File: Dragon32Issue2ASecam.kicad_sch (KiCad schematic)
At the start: 1 part

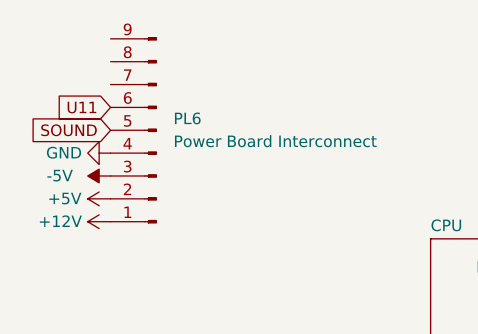
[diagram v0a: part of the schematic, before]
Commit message: fm circuit routing
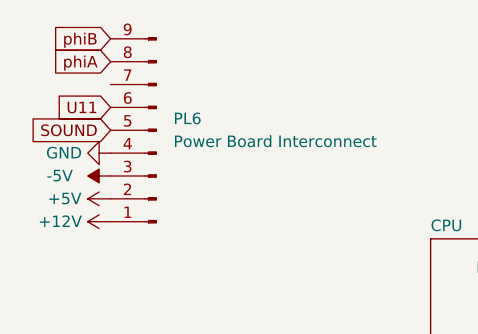
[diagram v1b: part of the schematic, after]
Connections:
- net phiA: now reaches PL6.8 (Pin_8)
- net phiB: now reaches PL6.9 (Pin_9)
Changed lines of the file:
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@@
+		)
+	)
+	(global_label "phiB"
+		(shape input)
+		(at 33.02 22.86 180)
+		(fields_autoplaced yes)
+		(effects
+			(font
+				(size 1.27 1.27)
+			)
+			(justify right)
+		)
+		(property "Intersheetrefs" "${INTERSHEET_REFS}"
+			(at 25.862 22.86 0)
+			(effects
+				(font
+					(size 1.27 1.27)
+				)
+				(justify right)
+				(hide yes)
+			)
 		)
 	)
@@
 			(effects
 				(font
+					(size 1.27 1.27)
+				)
+				(justify right)
+				(hide yes)
+			)
+		)
+	)
+	(global_label "phiA"
+		(shape input)
+		(at 33.02 25.4 180)
+		(fields_autoplaced yes)
+		(effects
+			(font
+				(size 1.27 1.27)
+			)
+			(justify right)
+		)
+		(property "Intersheetrefs" "${INTERSHEET_REFS}"
+			(at 26.0434 25.4 0)
+			(effects
+				(font

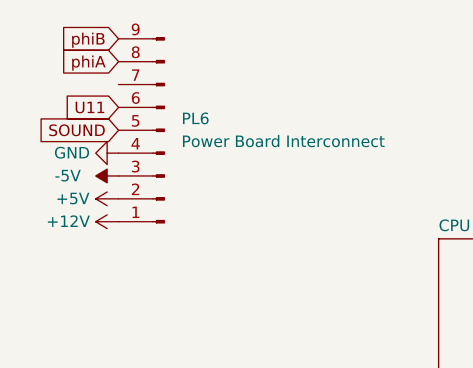
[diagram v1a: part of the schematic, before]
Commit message: trace work complete
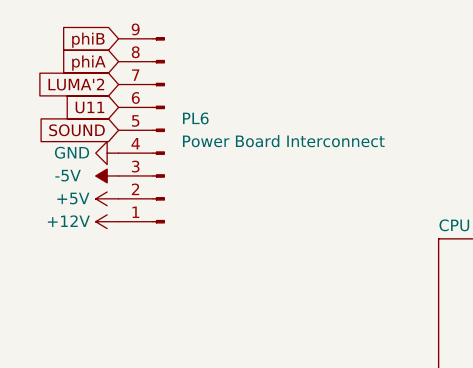
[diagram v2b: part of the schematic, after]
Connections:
- net LUMA'2: now reaches PL6.7 (Pin_7)
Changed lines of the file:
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@@
+		)
+	)
+	(global_label "LUMA'2"
+		(shape input)
+		(at 33.02 27.94 180)
+		(fields_autoplaced yes)
+		(effects
+			(font
+				(size 1.27 1.27)
+			)
+			(justify right)
+		)
+		(property "Intersheetrefs" "${INTERSHEET_REFS}"
+			(at 23.3219 27.94 0)
+			(effects
+				(font
+					(size 1.27 1.27)
+				)
+				(justify right)
+				(hide yes)
+			)
 		)
 	)
